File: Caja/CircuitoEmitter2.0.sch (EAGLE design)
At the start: 8 parts

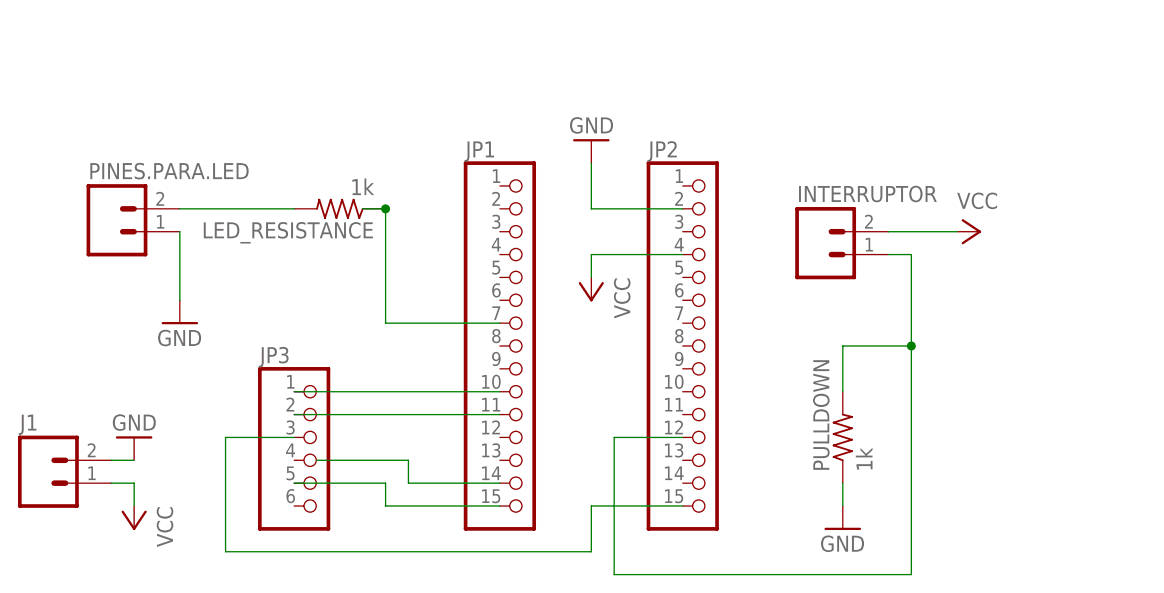
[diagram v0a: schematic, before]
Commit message: Modelo Final PCB Boton node
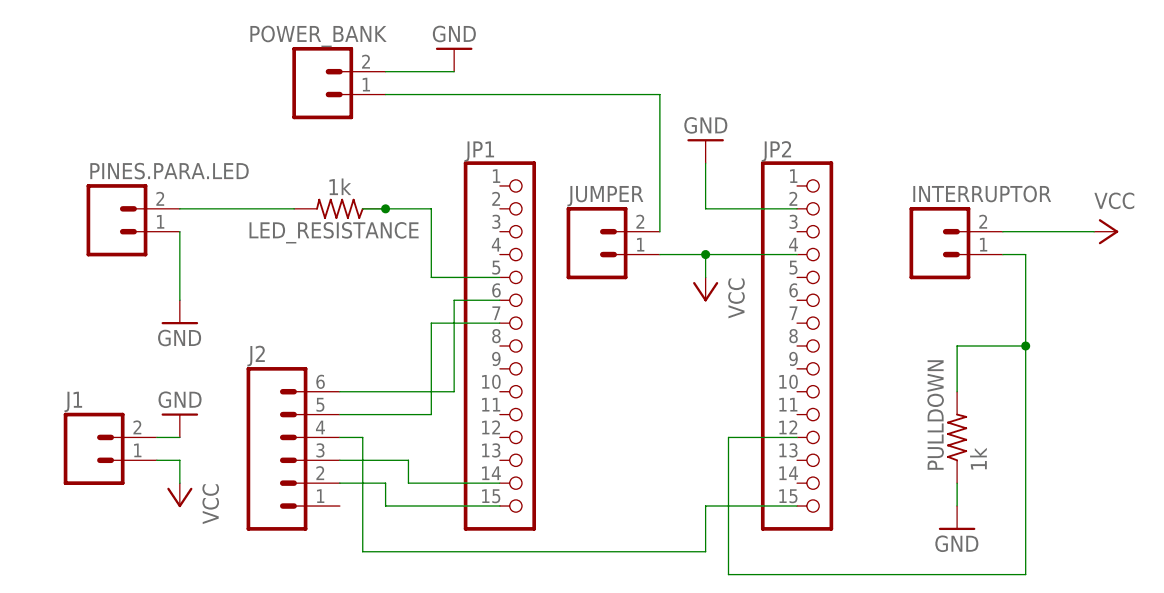
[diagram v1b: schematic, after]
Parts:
- removed JP3: (no value), adafruit:PINHD-1X6CLEAN
- added J2: (no value), mecatronica_eagle_lib:M06LONGPADS
- added JUMPER, POWER_BANK: (no value), mecatronica_eagle_lib:M02LOCK_LONGPADS
- J1: device mecatronica_eagle_lib:M02POGO_PIN_HOLES_ONLY -> mecatronica_eagle_lib:M02LOCK_LONGPADS
- JP1, JP2: device adafruit:PINHD-1X15-CB -> adafruit:PINHD-1X15
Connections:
- removed net N$2: JP1.11, JP3.2
- new net N$10: J2.6, JP1.6
- new net N$7: JUMPER.2, POWER_BANK.1
- net GND: now also POWER_BANK.2
- net N$1: now also J2.5, JP1.7; no longer JP1.10, JP3.1
- net N$3: now also J2.4; no longer JP3.3
- net N$4: now also J2.3
- net N$5: now also J2.2; no longer JP3.5
- net N$9: now also JP1.5; no longer JP1.7
- net VCC: now also JUMPER.1
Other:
- moved on the sheet: INTERRUPTOR, J1, JP2, PULLDOWN
